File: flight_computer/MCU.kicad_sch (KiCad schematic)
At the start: 30 parts, among them J1 Conn_02x05_Odd_Even, J2 MEM2061-01-188-00-A_REVA, Q1 Q_NPN_BEC, SW1 SW_Push, SW2 SW_Push, U2 STM8S007C8T6TR, Y1 12MHz

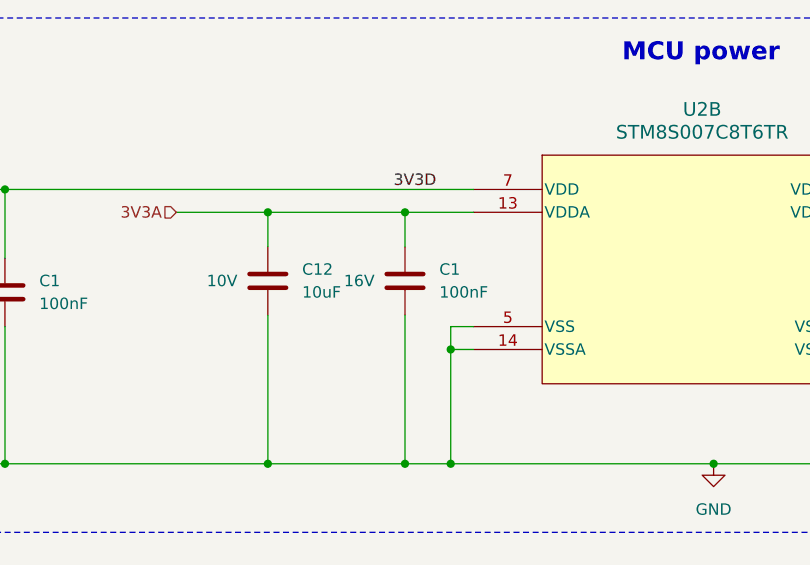
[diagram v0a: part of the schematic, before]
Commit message: Start of layout
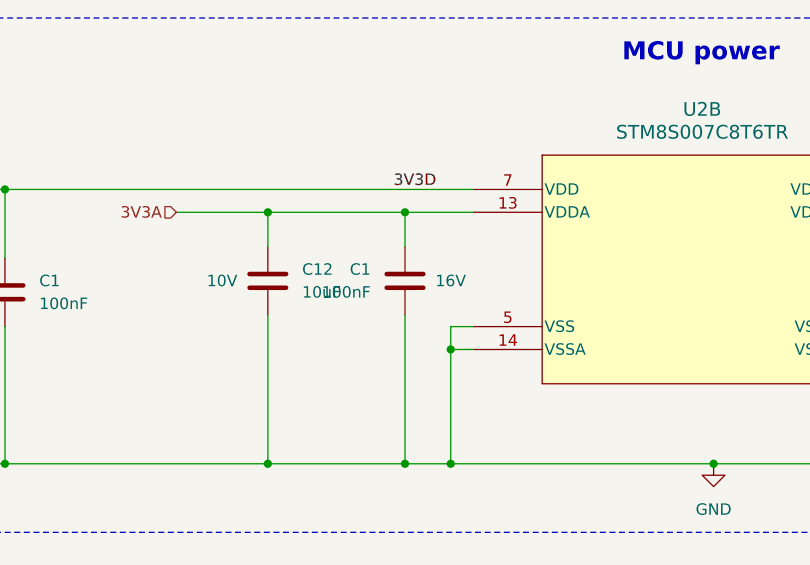
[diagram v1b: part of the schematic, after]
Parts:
- C12: footprint Capacitor_SMD:C_0201_0603Metric -> Capacitor_SMD:C_0402_1005Metric
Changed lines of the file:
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@@
       (effects (font (size 1.27 1.27)) (justify left))
     )
-    (property "Footprint" "Capacitor_SMD:C_0201_0603Metric" (at 122.8852 53.34 0)
+    (property "Footprint" "Capacitor_SMD:C_0402_1005Metric" (at 122.8852 53.34 0)
       (effects (font (size 1.27 1.27)) hide)
     )
@@
     )
   )
-  (symbol (lib_id "Device:C") (at 137.16 49.53 0) (unit 1)
-    (in_bom yes) (on_board yes) (dnp no)
-    (property "Reference" "C1" (at 140.97 48.26 0)
-      (effects (font (size 1.27 1.27)) (justify left))
-    )
-    (property "Value" "100nF" (at 140.97 50.8 0)
-      (effects (font (size 1.27 1.27)) (justify left))
-    )
-    (property "Footprint" "Capacitor_SMD:C_0402_1005Metric" (at 138.1252 53.34 0)
+  (symbol (lib_id "Device:C") (at 137.16 49.53 0) (mirror y) (unit 1)
+    (in_bom yes) (on_board yes) (dnp no)
+    (property "Reference" "C1" (at 133.35 48.26 0)
+      (effects (font (size 1.27 1.27)) (justify left))
+    )
+    (property "Value" "100nF" (at 133.35 50.8 0)
+      (effects (font (size 1.27 1.27)) (justify left))
+    )
+    (property "Footprint" "Capacitor_SMD:C_0402_1005Metric" (at 136.1948 53.34 0)
       (effects (font (size 1.27 1.27)) hide)
     )
@@
       (effects (font (size 1.27 1.27)) hide)
     )
-    (property "Voltage" "16V" (at 132.08 49.53 0)
+    (property "Voltage" "16V" (at 142.24 49.53 0)
       (effects (font (size 1.27 1.27)))
     )
@@
       (effects (font (size 1.27 1.27)) (justify left))
     )
-    (property "Footprint" "Capacitor_SMD:C_0201_0603Metric" (at 253.6952 50.8 0)
+    (property "Footprint" "Capacitor_SMD:C_0402_1005Metric" (at 253.6952 50.8 0)
       (effects (font (size 1.27 1.27)) hide)
     )
@@
       (effects (font (size 1.27 1.27)) (justify left))
     )
-    (property "Footprint" "Capacitor_SMD:C_0201_0603Metric" (at 74.6252 54.61 0)
+    (property "Footprint" "Capacitor_SMD:C_0402_1005Metric" (at 74.6252 54.61 0)
       (effects (font (size 1.27 1.27)) hide)
     )
@@
       (effects (font (size 1.27 1.27)) (justify left))
     )
-    (property "Footprint" "Capacitor_SMD:C_0201_0603Metric" (at 270.2052 50.8 0)
-      (effects (font (size 1.27 1.27)) hide)
-    )
+    (property "Footprint" "Capacitor_SMD:C_0402_1005Metric" (at 270.2052 50.8 0)
+      (effects (font (size 1.27 1.27)) hide)
+    )

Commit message: Layout first effort done
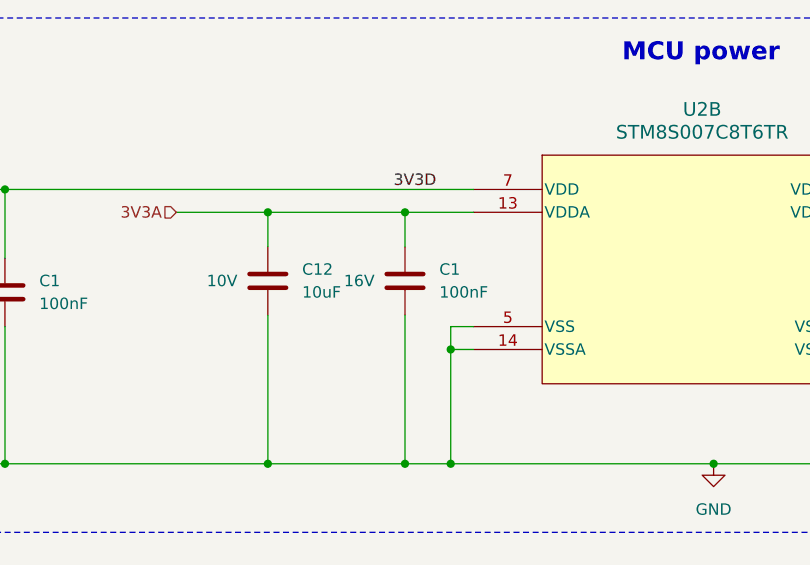
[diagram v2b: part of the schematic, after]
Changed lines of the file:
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@@
     )
   )
-  (symbol (lib_id "Device:C") (at 137.16 49.53 0) (mirror y) (unit 1)
+  (symbol (lib_id "Device:C") (at 137.16 49.53 0) (unit 1)
     (in_bom yes) (on_board yes) (dnp no)
-    (property "Reference" "C1" (at 133.35 48.26 0)
+    (property "Reference" "C1" (at 140.97 48.26 0)
       (effects (font (size 1.27 1.27)) (justify left))
     )
-    (property "Value" "100nF" (at 133.35 50.8 0)
+    (property "Value" "100nF" (at 140.97 50.8 0)
       (effects (font (size 1.27 1.27)) (justify left))
     )
-    (property "Footprint" "Capacitor_SMD:C_0402_1005Metric" (at 136.1948 53.34 0)
+    (property "Footprint" "Capacitor_SMD:C_0402_1005Metric" (at 138.1252 53.34 0)
       (effects (font (size 1.27 1.27)) hide)
     )
@@
       (effects (font (size 1.27 1.27)) hide)
     )
-    (property "Voltage" "16V" (at 142.24 49.53 0)
+    (property "Voltage" "16V" (at 132.08 49.53 0)
       (effects (font (size 1.27 1.27)))
     )
